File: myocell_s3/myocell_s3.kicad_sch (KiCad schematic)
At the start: 6 parts, among them J1 Conn_01x08, J2 Conn_01x08, J3 Conn_01x08, J4 Conn_01x08, J5 Battery Connector JC2, J7 USB_C_Receptacle_USB2.0_16P

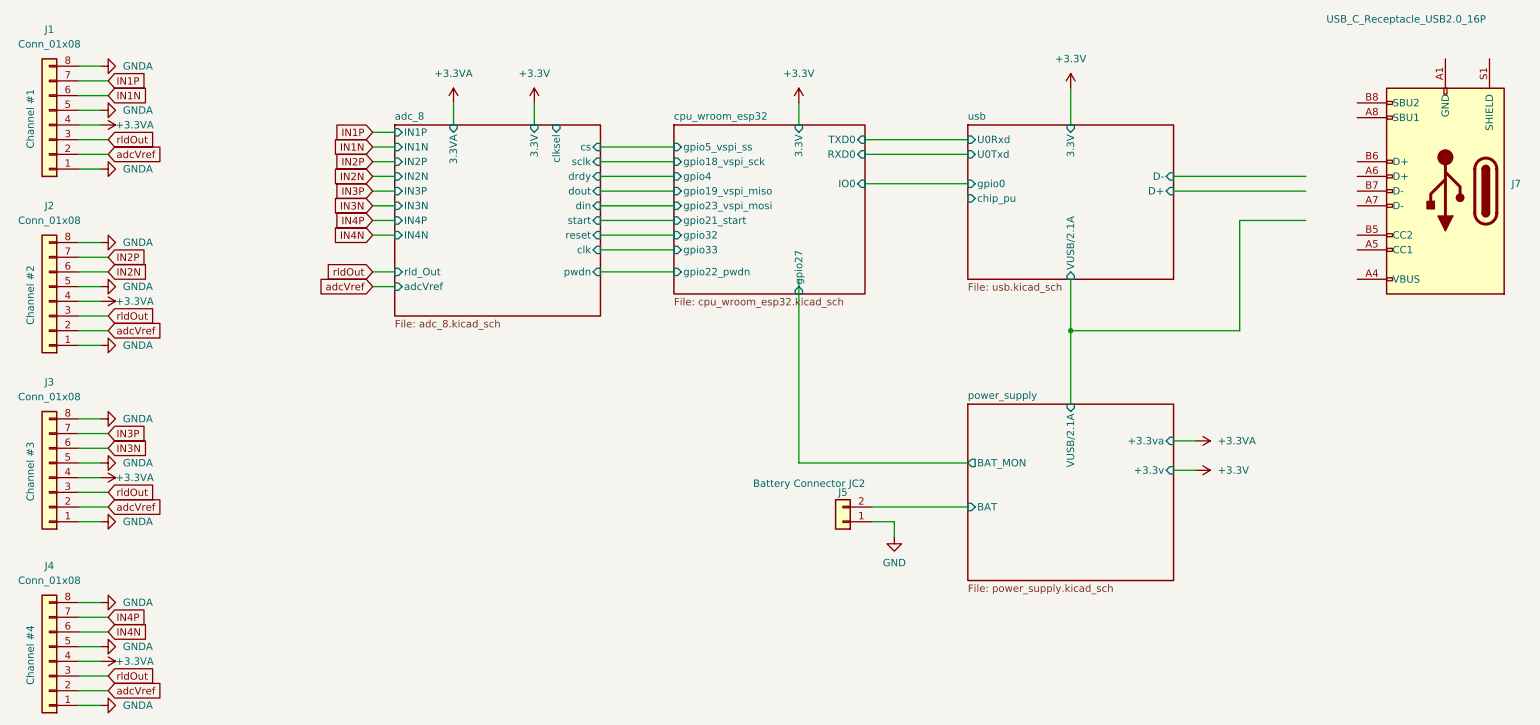
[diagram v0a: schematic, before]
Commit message: working on schematic
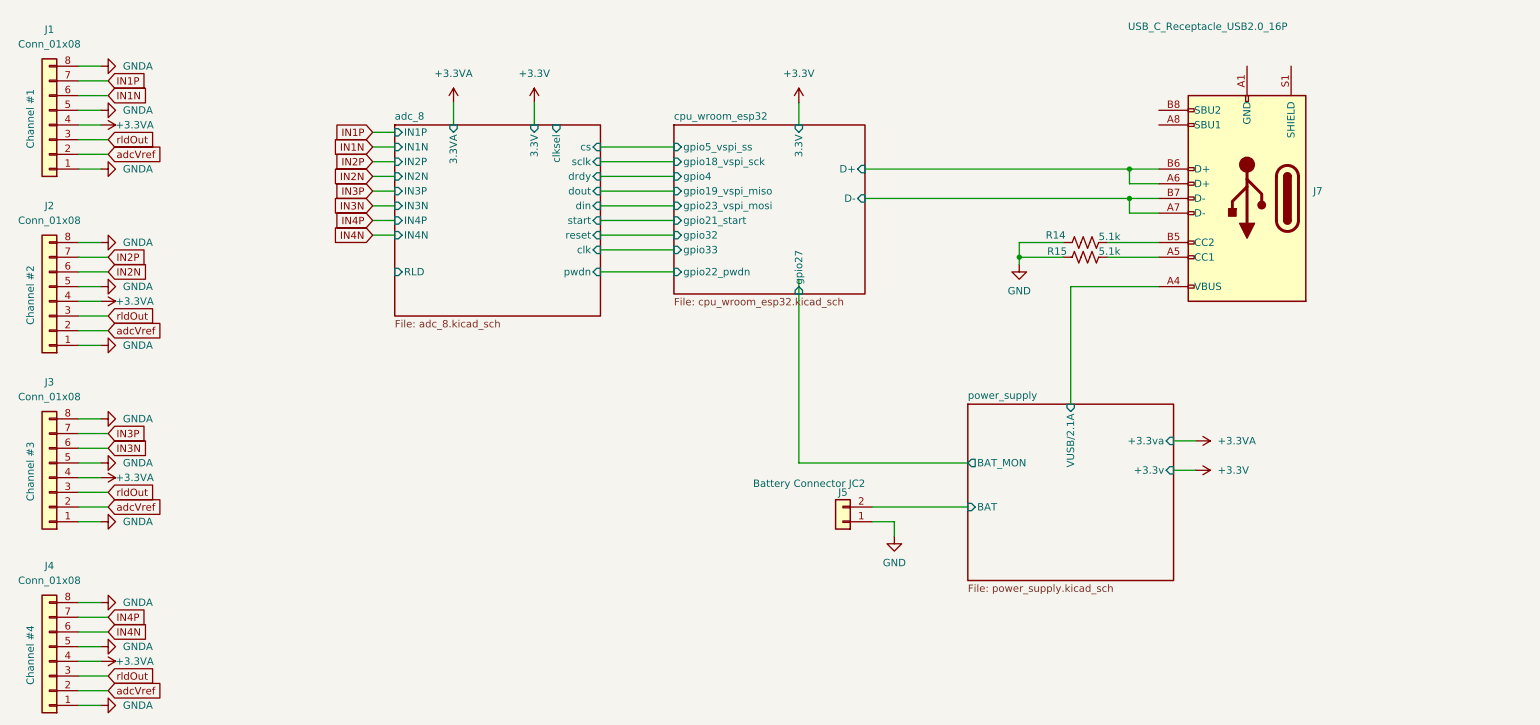
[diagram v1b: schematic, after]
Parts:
- added R14, R15: 5.1k, Resistor_SMD:R_0805_2012Metric_Pad1.20x1.40mm_HandSolder, symbol Device:R_US
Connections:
- net GND: now also R14.1, R15.1
- net power_supply/VUSB/2.1A: now also J7.A4 (VBUS), J7.A9 (VBUS), J7.B4 (VBUS), J7.B9 (VBUS)
- net at J7.A5 (CC1): now also R15.2
- net cpu_wroom_esp32/D+: now reaches J7.A6 (D+)
- net cpu_wroom_esp32/D+: now also J7.B6 (D+)
- net cpu_wroom_esp32/D-: now reaches J7.A7 (D-)
- net cpu_wroom_esp32/D-: now also J7.B7 (D-)
- net at J7.B5 (CC2): now also R14.2
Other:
- removed sheet usb
- sheet adc_8 ports: added RLD; removed adcVref, rld_Out
- sheet cpu_wroom_esp32 ports: added D+, D-; removed IO0, RXD0, TXD0
- moved on the sheet: J7

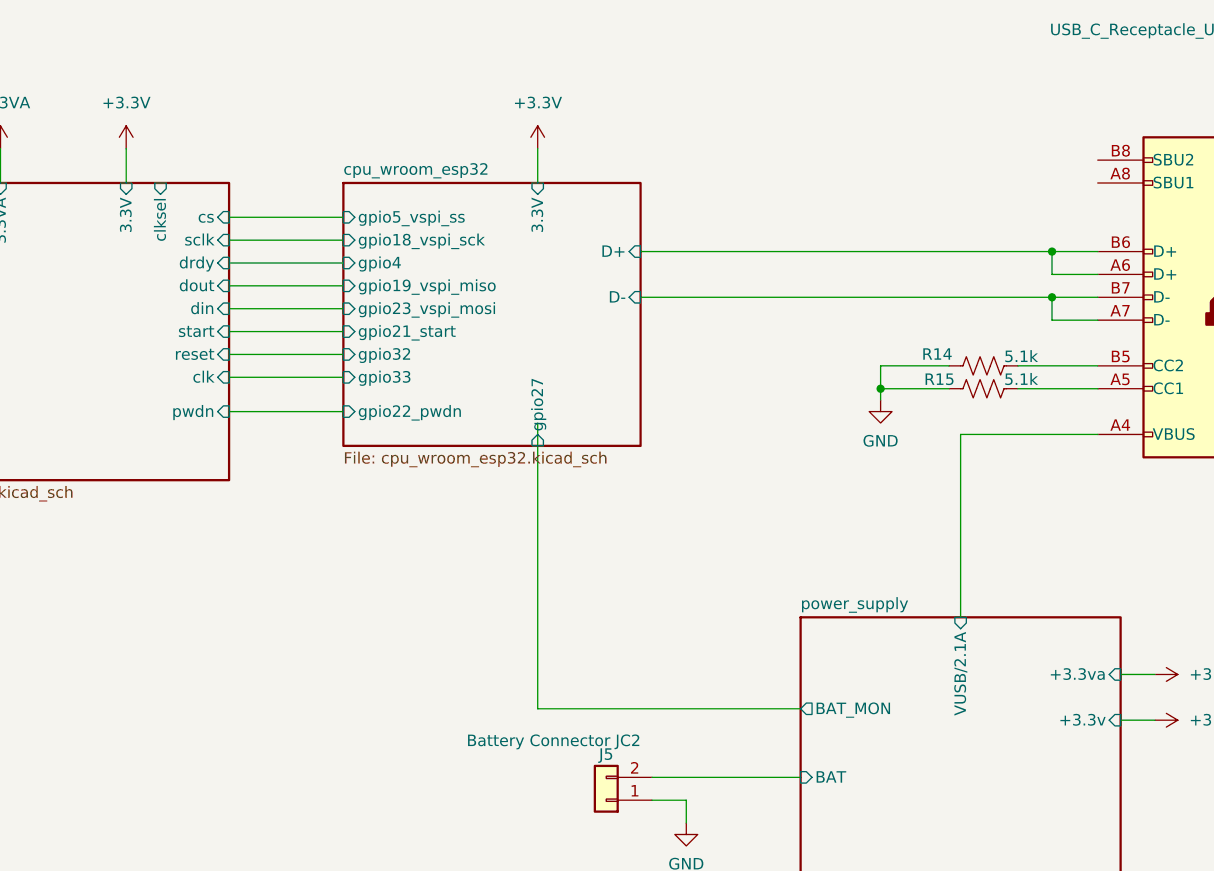
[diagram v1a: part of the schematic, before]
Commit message: working on schematic
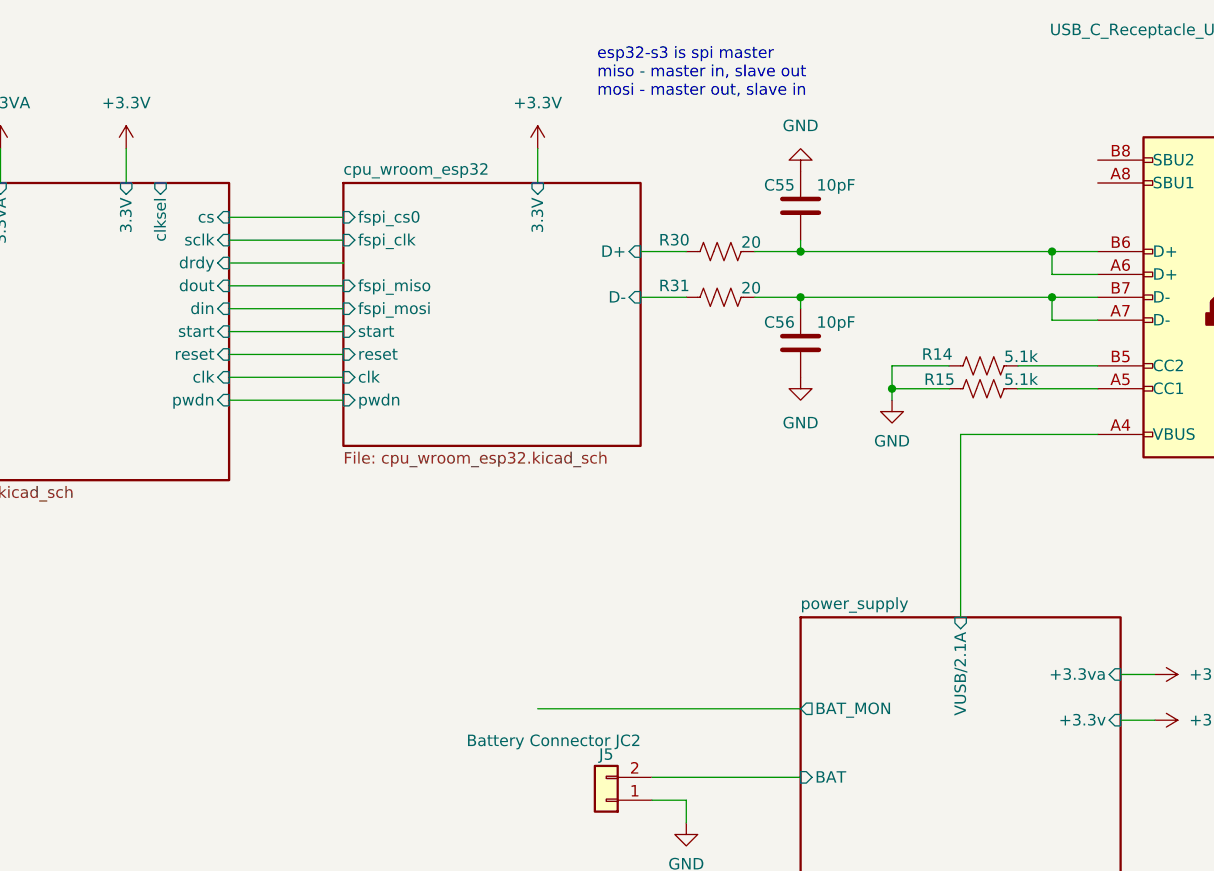
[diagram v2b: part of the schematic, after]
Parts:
- added C55, C56: 10pF, Capacitor_SMD:C_0805_2012Metric_Pad1.18x1.45mm_HandSolder, symbol Device:C
- added R30, R31: 20, Resistor_SMD:R_0805_2012Metric_Pad1.20x1.40mm_HandSolder, symbol Device:R_US
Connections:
- net GND: now also C55.1, C56.2
- net cpu_wroom_esp32/D+: now also R30.1; no longer J7.A6 (D+), J7.B6 (D+)
- net cpu_wroom_esp32/D-: now also R31.1; no longer J7.A7 (D-), J7.B7 (D-)
- new net: C55.2, J7.A6 (D+), J7.B6 (D+), R30.2
- new net: C56.1, J7.A7 (D-), J7.B7 (D-), R31.2
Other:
- sheet cpu_wroom_esp32 ports: added clk, fspi_clk, fspi_cs0, fspi_miso, fspi_mosi, pwdn, reset, start; removed gpio18_vspi_sck, gpio19_vspi_miso, gpio21_start, gpio22_pwdn, gpio23_vspi_mosi, gpio27, gpio32, gpio33, gpio4, gpio5_vspi_ss
- note added: "esp32-s3 is spi master miso - master in, slave out mosi - master out, slave in"
